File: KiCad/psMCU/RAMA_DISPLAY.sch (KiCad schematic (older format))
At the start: 9 parts

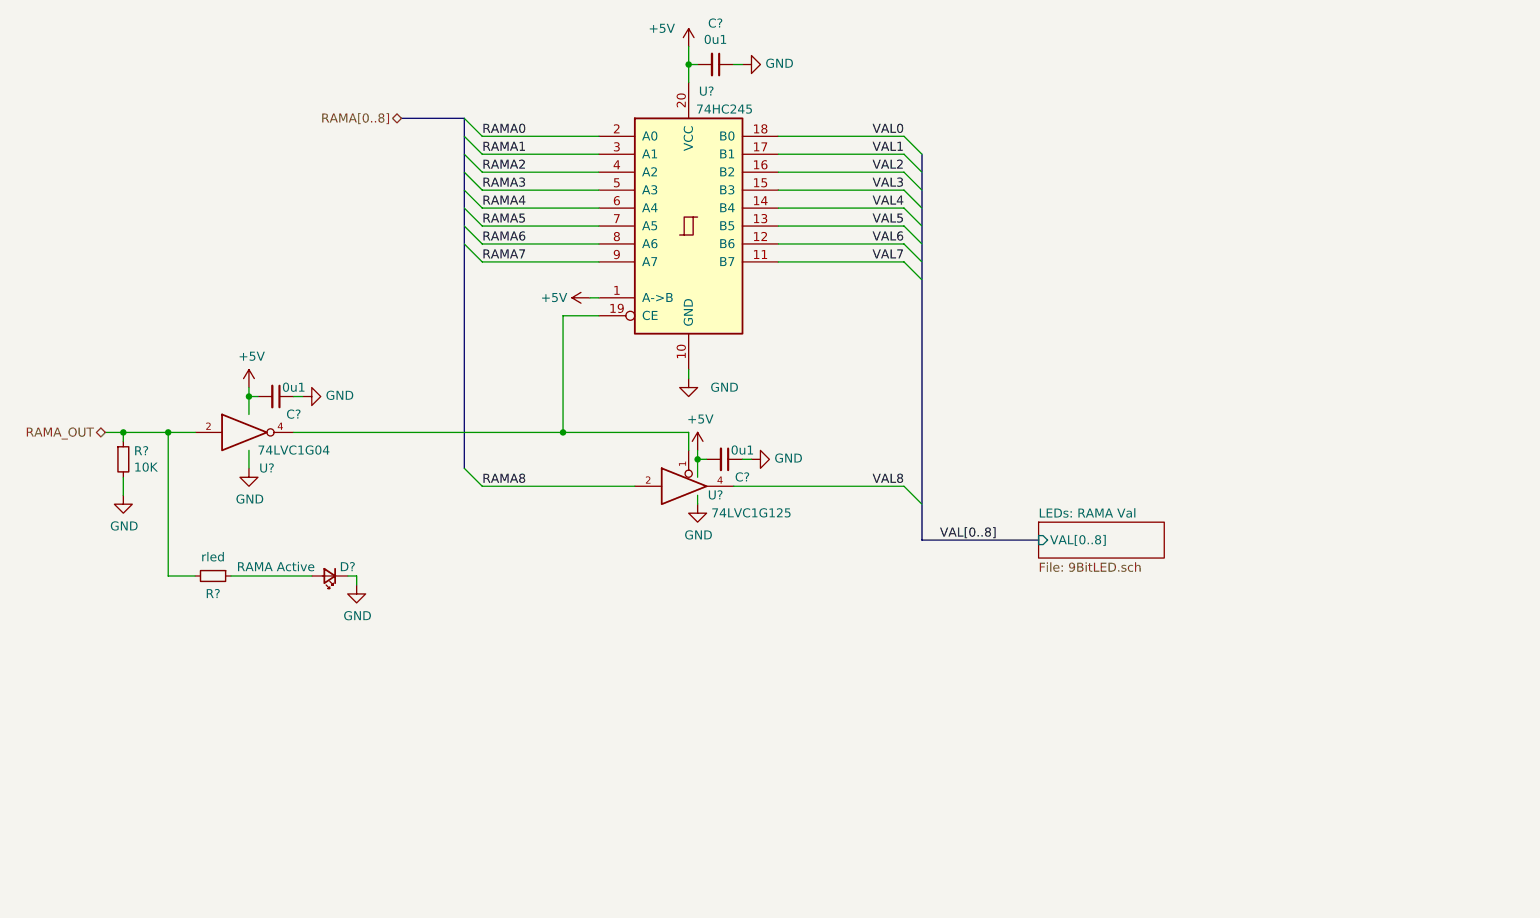
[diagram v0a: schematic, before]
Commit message: First Schematic Draft done.
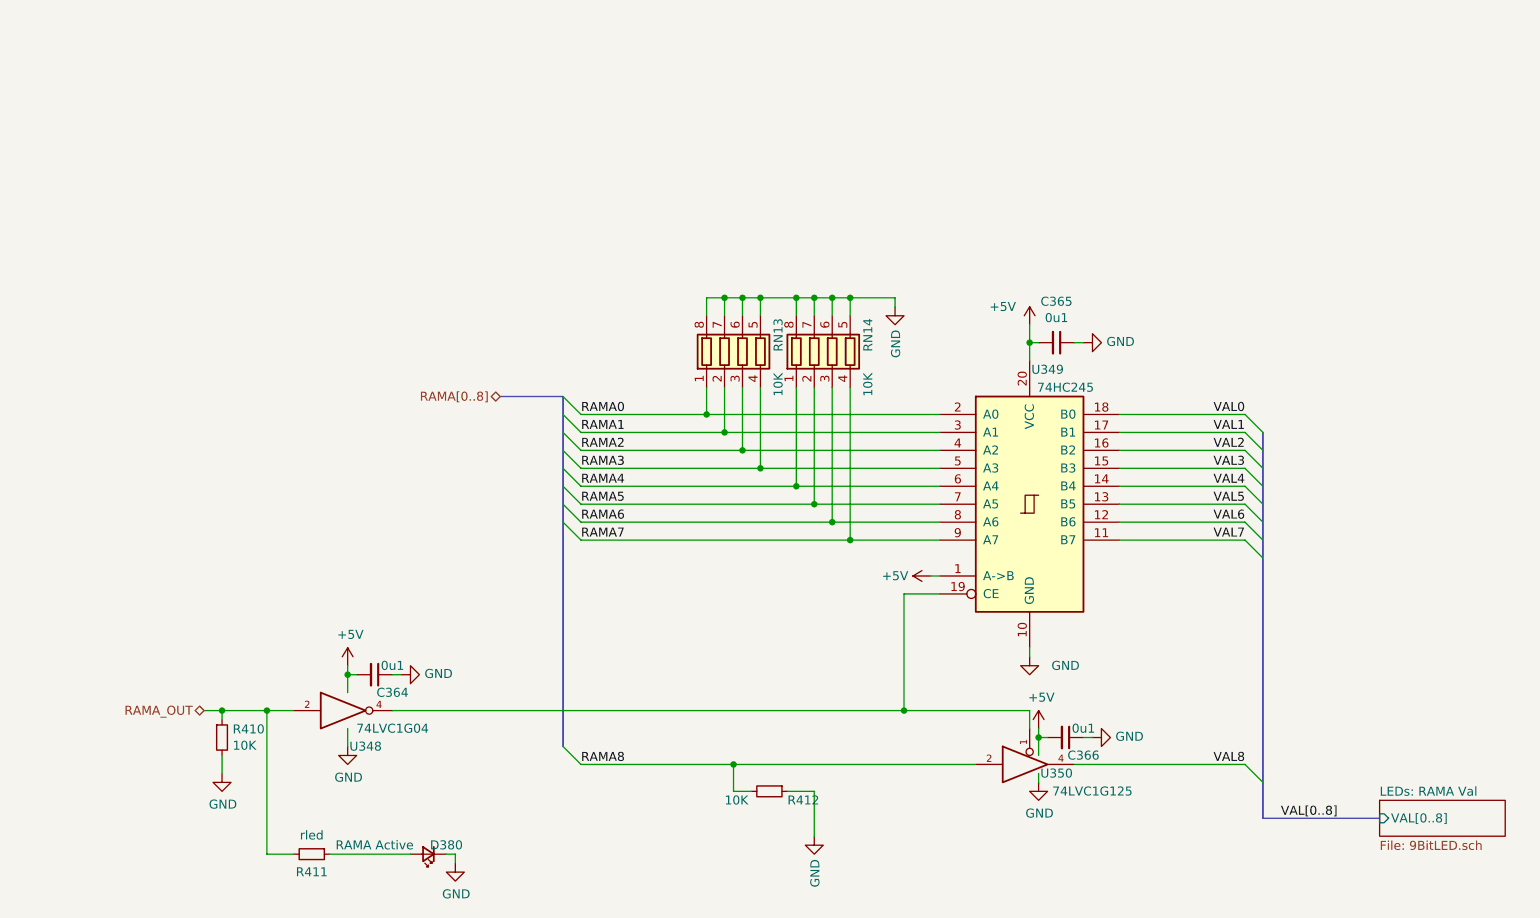
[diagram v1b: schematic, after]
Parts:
- added R412: 10K, symbol Device:R_Small
- added RN13, RN14: 10K, Resistor_SMD:R_Array_Convex_4x0603, symbol Device:R_Pack04
- C364, C365, C366: renamed from C?; footprint Capacitor_SMD:C_0603_1608Metric -> NoRef_Footprints:C_0603_1608Metric_NoRef
- D380: renamed from D?; footprint Diode_SMD:D_0603_1608Metric -> NoRef_Footprints:D_0603_1608Metric_NoRef
- R410: renamed from R?; footprint Resistor_SMD:R_0603_1608Metric -> NoRef_Footprints:D_0603_1608Metric_NoRef
- R411: renamed from R?; footprint Resistor_SMD:R_0603_1608Metric -> NoRef_Footprints:R_0603_1608Metric
- gave numbers to parts that had none: 3
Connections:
- net GND: now also R412.1, RN13.5 (R4.2), RN13.6 (R3.2), RN13.7 (R2.2), RN13.8 (R1.2), RN14.5 (R4.2), RN14.6 (R3.2), RN14.7 (R2.2), RN14.8 (R1.2)
- net RAMA0: now also RN13.1 (R1.1)
- net RAMA1: now also RN13.2 (R2.1)
- net RAMA2: now also RN13.3 (R3.1)
- net RAMA3: now also RN13.4 (R4.1)
- net RAMA4: now also RN14.1 (R1.1)
- net RAMA5: now also RN14.2 (R2.1)
- net RAMA6: now also RN14.3 (R3.1)
- net RAMA7: now also RN14.4 (R4.1)
- net RAMA8: now also R412.2
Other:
- moved on the sheet: C364, C365, C366, D380, R410, R411, U348, U349, U350
